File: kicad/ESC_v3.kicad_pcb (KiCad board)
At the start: 4 copper layers, 50 x 50 mm, 175 parts, among them J1 Conn_01x05_Pin, J2 Conn_01x05_Pin, J3 Conn_01x01_Pin, J4 Conn_01x06_Pin, J5 Conn_01x02_Pin, J6 Conn_01x06_Pin, J7 Conn_01x02_Pin, J8 Conn_01x04_Pin, J9 Conn_01x02_Pin, Q1 RH6L040BGTB1, Q10 RH6L040BGTB1, Q11 RH6L040BGTB1, Q12 RH6L040BGTB1, Q2 RH6L040BGTB1, Q3 RH6L040BGTB1, Q4 RH6L040BGTB1, Q5 RH6L040BGTB1, Q6 RH6L040BGTB1, Q7 RH6L040BGTB1, Q8 RH6L040BGTB1, Q9 RH6L040BGTB1, SW2 SW_Nidec_CAS-120A1, U1 L6387, U10 BD4104, U11 AMS1117-5.0, U12 ACS711xEXLT-15AB, U13 LM2937xMP, U14 MCP9700x-ETT, U15 MAX40200AUK, U19 STM32G431CBUx, U2 L6387, U3 L6387, U4 L6387, U5 L6387, U6 L6387, U7 AMS1117-3.3, U8 ACS711xEXLT-15AB, U9 ACS711xEXLT-15AB

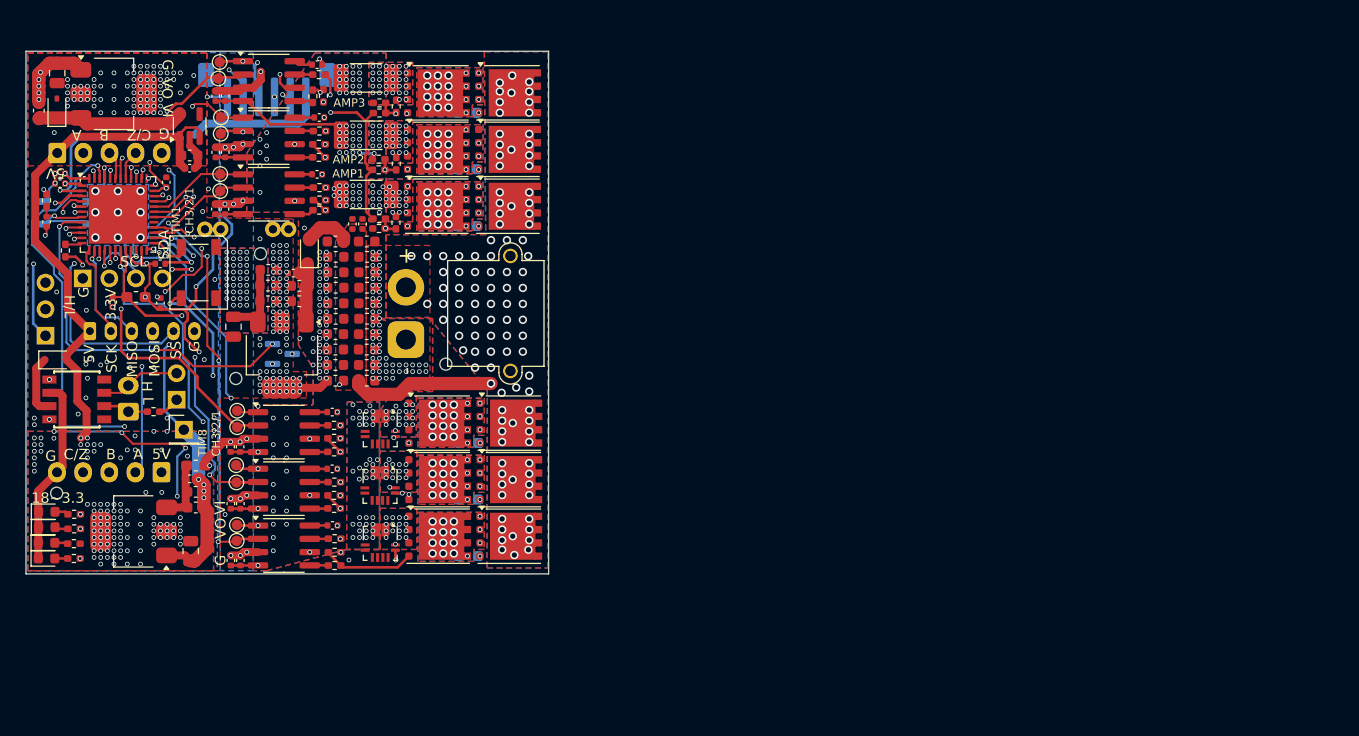
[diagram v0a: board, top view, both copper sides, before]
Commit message: a
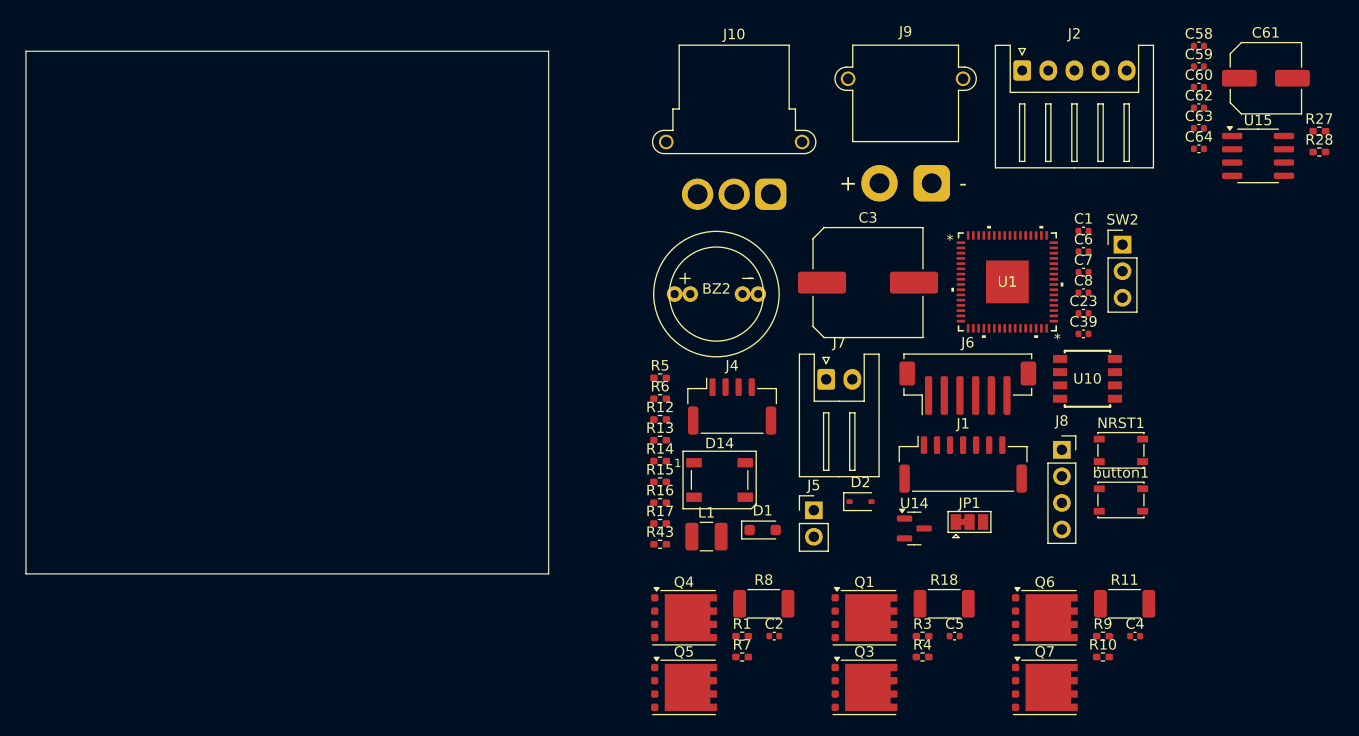
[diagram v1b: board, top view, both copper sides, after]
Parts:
- removed BZ1: Buzzer, jisaku:buzzer_unified
- removed C10, C12, C13, C15, C16, C18, C32, C38, C9: 0.1u, Capacitor_SMD:C_0402_1005Metric
- removed C11, C14, C17, C21, C33, C34, C35, C36, C37: 1u, Capacitor_SMD:C_0402_1005Metric
- removed C19, C20, C22: 10u, Capacitor_SMD:C_0603_1608Metric
- removed C24, C31, C40, C41, C42, C43, C44, C45, C46, C47, C48, C49, C50, C51, C52, C53, C54, C55, C56, C57: 22uF, Capacitor_SMD:C_0603_1608Metric
- removed C25, C29: 10uF, Capacitor_SMD:C_0603_1608Metric
- removed C26, C28, C30: 22uF, Capacitor_SMD:C_0805_2012Metric
- removed C27: 0.47uF, Capacitor_SMD:C_0603_1608Metric
- removed D13, D15, D16, D17: LED, LED_SMD:LED_0603_1608Metric
- removed D3: 1N5819WS, Diode_SMD:D_SOD-323
- removed G***: LOGO, agazou:full
- removed G***: LOGO, agazou:drive
- removed G***: LOGO, agazou:core
- removed G***: LOGO, agazou:blackpulsedrive
- removed J3: Conn_01x01_Pin, Connector_PinHeader_2.54mm:PinHeader_1x01_P2.54mm_Vertical
- removed L3: L, Inductor_SMD:L_0603_1608Metric_Pad1.05x0.95mm_HandSolder
- removed Q10, Q11, Q12, Q2, Q8, Q9: RH6L040BGTB1, Package_SON:VSONP-8-1EP_5x6_P1.27mm
- removed R19, R2, R20, R23, R24: 22, Resistor_SMD:R_0402_1005Metric_Pad0.72x0.64mm_HandSolder
- removed R21, R25, R57: 10k, Resistor_SMD:R_0402_1005Metric_Pad0.72x0.64mm_HandSolder
- removed R22, R26: 10k, Resistor_SMD:R_0603_1608Metric_Pad0.98x0.95mm_HandSolder
- removed R29: 100, Resistor_SMD:R_0402_1005Metric_Pad0.72x0.64mm_HandSolder
- removed R44, R45, R51: 5m, Resistor_SMD:R_2010_5025Metric_Pad1.40x2.65mm_HandSolder
- removed R46, R47, R52: 1.5k, Resistor_SMD:R_0402_1005Metric_Pad0.72x0.64mm_HandSolder
- removed R48, R49, R54: 68k, Resistor_SMD:R_0402_1005Metric_Pad0.72x0.64mm_HandSolder
- removed R50, R53, R55, R59: 2.2k, Resistor_SMD:R_0402_1005Metric_Pad0.72x0.64mm_HandSolder
- removed R56: 22k, Resistor_SMD:R_0402_1005Metric_Pad0.72x0.64mm_HandSolder
- removed R58: 4.7k, Resistor_SMD:R_0402_1005Metric_Pad0.72x0.64mm_HandSolder
- removed REF** (x4): ToolingHole_1.152mm, MountingHole:ToolingHole_1.152mm
- removed TP1, TP10, TP11, TP12, TP2, TP3, TP4, TP5, TP6, TP7, TP8, TP9: TestPoint, TestPoint:TestPoint_Pad_D1.0mm
- removed U11: AMS1117-5.0, Package_TO_SOT_SMD:SOT-223-3_TabPin2
- removed U12, U8, U9: ACS711xEXLT-15AB, Sensor_Current:Allegro_QFN-12-10-1EP_3x3mm_P0.5mm
- removed U13: LM2937xMP, Package_TO_SOT_SMD:SOT-223-3_TabPin2
- removed U19: STM32G431CBUx, Package_DFN_QFN:QFN-48-1EP_7x7mm_P0.5mm_EP5.6x5.6mm
- removed U2, U3, U4, U5, U6: L6387, Package_SO:SOIC-8_3.9x4.9mm_P1.27mm
- removed U7: AMS1117-3.3, Package_TO_SOT_SMD:SOT-223-3_TabPin2
- added BZ2: Buzzer, jisaku:buzzer_unified, F.Cu at (116.1, 73.2)
- added C39: 0.1u, Capacitor_SMD:C_0402_1005Metric, F.Cu at (151.2, 77.0)
- added C64: 10u, Capacitor_SMD:C_0402_1005Metric, F.Cu at (162.2, 59.3)
- added J10: Conn_01x03, Connector_AMASS:AMASS_MR30PW-FB_1x03_P3.50mm_Horizontal, F.Cu at (121.3, 63.7)
- added JP1: SolderJumper_3_Bridged12, Jumper:SolderJumper-3_P1.3mm_Bridged12_Pad1.0x1.5mm, F.Cu at (140.3, 95.0)
- added R27: 10k, Resistor_SMD:R_0402_1005Metric_Pad0.72x0.64mm_HandSolder, F.Cu at (173.7, 57.6)
- added R28: 10, Resistor_SMD:R_0402_1005Metric_Pad0.72x0.64mm_HandSolder, F.Cu at (173.7, 59.6)
- added R5: 10k, Resistor_SMD:R_0402_1005Metric_Pad0.72x0.64mm_HandSolder, F.Cu at (110.7, 81.2)
- added button1: SW_Push, Button_Switch_SMD:SW_SPST_PTS810, F.Cu at (154.8, 92.9)
- C1, C6, C7: value 0.1u -> 10u
- C3: value 0.1u -> 470u; footprint Capacitor_SMD:C_0402_1005Metric -> Capacitor_SMD:C_Elec_10x10.2
- C4: value 0.1u -> 1u
- C58: value 100u -> 4.7u; footprint Capacitor_SMD:C_0603_1608Metric -> Capacitor_SMD:C_0402_1005Metric
- C59: value 0.1u -> 0.033u
- C60: value 100u -> 0.05u; footprint Capacitor_SMD:C_0603_1608Metric -> Capacitor_SMD:C_0402_1005Metric
- C61: value 0.1u -> 470u; footprint Capacitor_SMD:C_0402_1005Metric -> Capacitor_SMD:C_Elec_6.3x7.7
- C62: value 100u -> 10u; footprint Capacitor_SMD:C_0603_1608Metric -> Capacitor_SMD:C_0402_1005Metric
- C8: value 1u -> 10u
- D1: value 1N5819WS -> D; footprint Diode_SMD:D_SOD-323 -> Diode_SMD:D_SOD-323_HandSoldering
- J1: value Conn_01x05_Pin -> Conn_01x07; footprint Connector_JST:JST_XH_S5B-XH-A_1x05_P2.50mm_Horizontal -> Connector_JST:JST_GH_SM07B-GHS-TB_1x07-1MP_P1.25mm_Horizontal; moved to F.Cu
- J2, J5, J6, J7, J8, NRST1, SW2, U14: moved to F.Cu
- J4: value Conn_01x06_Pin -> Conn_01x04; footprint Connector_JST:JST_PH_B6B-PH-K_1x06_P2.00mm_Vertical -> Connector_JST:JST_GH_SM04B-GHS-TB_1x04-1MP_P1.25mm_Horizontal; moved to F.Cu
- J9: value Conn_01x02_Pin -> Conn_01x02
- L1: value L -> 10uH; footprint Inductor_SMD:L_0603_1608Metric_Pad1.05x0.95mm_HandSolder -> Inductor_SMD:L_1210_3225Metric
- R1, R12, R15, R16, R7: value 22 -> R
- R10, R14, R4: value 10k -> R; footprint Resistor_SMD:R_0603_1608Metric_Pad0.98x0.95mm_HandSolder -> Resistor_SMD:R_0402_1005Metric_Pad0.72x0.64mm_HandSolder; moved to F.Cu
- R11, R8: value 22 -> R; footprint Resistor_SMD:R_0402_1005Metric_Pad0.72x0.64mm_HandSolder -> Resistor_SMD:R_2010_5025Metric
- R13, R17, R3, R9: value 10k -> R
- R18: value 10k -> R; footprint Resistor_SMD:R_0603_1608Metric_Pad0.98x0.95mm_HandSolder -> Resistor_SMD:R_2010_5025Metric; moved to F.Cu
- U1: value L6387 -> STSPIN32G4; footprint Package_SO:SOIC-8_3.9x4.9mm_P1.27mm -> stspin32g4:QFN_IN32G4_STM
- U15: value MAX40200AUK -> LM386; footprint Package_TO_SOT_SMD:SOT-23-5 -> Package_SO:SOIC-8_3.9x4.9mm_P1.27mm
- moved NRST1 103.4 mm to (154.8, 88.2), turned to 0 degrees
- moved SW2 103.4 mm to (154.9, 68.5)
- moved C61 103.3 mm to (168.6, 52.6)
- moved C62 102.8 mm to (162.2, 55.4)
- moved U15 102.3 mm to (167.9, 60.0), turned to 0 degrees
- moved C63 102.2 mm to (162.2, 57.4)
- moved C23 99.6 mm to (151.2, 75.1), turned to 0 degrees
- moved C60 96.8 mm to (162.2, 53.4)
- moved U10 96.7 mm to (151.6, 81.3)
- moved J8 95.1 mm to (149.1, 88.1), turned to 0 degrees
- moved J1 91.6 mm to (139.7, 89.5)
- moved J2 90.9 mm to (145.3, 51.8), turned to 0 degrees
- moved R11 89.3 mm to (155.1, 102.9)
- moved C58 89.1 mm to (162.2, 49.5), turned to 0 degrees
- moved C59 88.9 mm to (162.2, 51.5), turned to 0 degrees
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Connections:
- C1 pad 1: +12V -> Net-(U1-VCC)
- C2 pad 1: +12V -> /power_stage1/BOOT
- C2 pad 2: GND -> /power_stage1/OUT
- C3 pad 1: Net-(U1-VB) -> +15V
- C3 pad 2: /POWER/halfHbridge4/out1 -> OPAMP3_VINM
- C4 pad 1: +12V -> /power_stage2/BOOT
- C4 pad 2: GND -> /power_stage2/OUT
- C5 pad 1: +12V -> /power_stage/BOOT
- C5 pad 2: GND -> /power_stage/OUT
- C58 pad 1: Net-(D1-K) -> DAC1_OUT1
- C58 pad 2: GND -> Net-(C58-Pad2)
- C59 pad 1: Net-(D1-K) -> Net-(C59-Pad1)
- C59 pad 2: GND -> Net-(C59-Pad2)
- C6 pad 1: Net-(U2-VB) -> Net-(U1-REG3V3/VDD)
- C6 pad 2: /POWER/halfHbridge5/out1 -> GND
- C60 pad 1: +5V -> Net-(C59-Pad1)
- C60 pad 2: GND -> Net-(C60-Pad2)
- C61 pad 1: +5V -> Net-(C59-Pad1)
- C61 pad 2: GND -> /Untitled Sheet/OUT
- C62 pad 1: Net-(U11-VI) -> Net-(U15-BYPASS)
- C63 pad 1: Net-(U11-VI) -> /Untitled Sheet/VDD
- C7 pad 1: +12V -> +5V
- C8 pad 1: +12V -> Net-(U1-VCC)
- D1 pad 2: VCC -> GND
- J1 pad 1: +5V -> +3.3V
- J1 pad 2: TIM3_CH1 -> ADC1_IN8
- J1 pad 3: TIM3_CH2 -> GND
- J1 pad 4: EXTI13 -> ADC1_IN7
- J1 pad 5: GND -> unconnected-(J1-Pin_5-Pad5)
- J2 pad 1: +5V -> Net-(J2-Pin_1)
- J2 pad 2: TIM2_CH1 -> CH1
- J2 pad 3: TIM2_CH2 -> CH2
- J2 pad 4: TIM2_CH3 -> CH3
- J4 pad 1: +5V -> +3.3V
- J4 pad 2: SPI1_SCK -> ADC1_IN8
- J4 pad 3: SPI1_MISO -> GND
- J4 pad 4: SPI1_MOSI -> ADC1_IN7
- J9 pad 1: GND -> +15V
- J9 pad 2: VCC -> OPAMP3_VINP
- L1 pad 1: +3.3V -> Net-(D1-K)
- L1 pad 2: VREF -> Net-(U1-VCC)
- Q1 pad 1: /POWER/halfHbridge4/out1 -> /power_stage/OUT
- Q1 pad 3: VCC -> /power_stage/Vm
- Q3 pad 1: /POWER/halfHbridge5/out1 -> /power_stage/OPAMP_P
- Q3 pad 3: VCC -> /power_stage/OUT
- Q4 pad 1: /POWER/halfHbridge5/GND_mech -> /power_stage1/OUT
- Q4 pad 3: /POWER/halfHbridge5/out1 -> /power_stage/Vm
- Q5 pad 1: /POWER/halfHbridge6/out1 -> /power_stage1/OPAMP_P
- Q5 pad 3: VCC -> /power_stage1/OUT
- Q6 pad 1: /POWER/halfHbridge6/GND_mech -> /power_stage2/OUT
- Q6 pad 3: /POWER/halfHbridge6/out1 -> /power_stage/Vm
- Q7 pad 1: /POWER/halfHbridge7/out1 -> /power_stage2/OPAMP_P
- Q7 pad 3: VCC -> /power_stage2/OUT
- R1 pad 1: Net-(U1-HO) -> /power_stage1/GHS
- R1 pad 2: Net-(Q1-G) -> Net-(Q4-G)
- R10 pad 1: Net-(Q3-G) -> /power_stage2/GLS
- R10 pad 2: /POWER/halfHbridge5/out1 -> Net-(Q7-G)
- R11 pad 1: Net-(U3-HO) -> /power_stage2/OPAMP_P
- R11 pad 2: Net-(Q5-G) -> OPAMP3_VINM
- R12 pad 1: Net-(U3-LO) -> /power_stage/OPAMP_P
- R12 pad 2: Net-(Q6-G) -> OPAMP1_VINP
- R13 pad 1: /POWER/halfHbridge6/GND_mech -> OPAMP1_VINP
- R13 pad 2: Net-(Q6-G) -> +3.3V
- R14 pad 1: Net-(Q5-G) -> GND
- R14 pad 2: /POWER/halfHbridge6/out1 -> OPAMP1_VINP
- R15 pad 1: Net-(U4-HO) -> /power_stage1/OPAMP_P
- R15 pad 2: Net-(Q7-G) -> OPAMP2_VINP
- R16 pad 1: Net-(U4-LO) -> OPAMP2_VINP
- R16 pad 2: Net-(Q8-G) -> +3.3V
- R17 pad 1: /POWER/halfHbridge7/GND_mech -> GND
- R17 pad 2: Net-(Q8-G) -> OPAMP2_VINP
- R18 pad 1: Net-(Q7-G) -> /power_stage/OPAMP_P
- R18 pad 2: /POWER/halfHbridge7/out1 -> OPAMP3_VINM
- R3 pad 1: /POWER/halfHbridge4/GND_mech -> /power_stage/GLS
- R3 pad 2: Net-(Q2-G) -> Net-(Q3-G)
- R4 pad 1: Net-(Q1-G) -> /power_stage/GHS
- R4 pad 2: /POWER/halfHbridge4/out1 -> Net-(Q1-G)
- R7 pad 1: Net-(U2-HO) -> /power_stage1/GLS
- R7 pad 2: Net-(Q3-G) -> Net-(Q5-G)
- R8 pad 1: Net-(U2-LO) -> /power_stage1/OPAMP_P
- R8 pad 2: Net-(Q4-G) -> OPAMP3_VINM
- R9 pad 1: /POWER/halfHbridge5/GND_mech -> /power_stage2/GHS
- R9 pad 2: Net-(Q4-G) -> Net-(Q6-G)
- U1 pad 1: TIM1_CH1 -> Net-(U1-REG3V3/VDD)
- U1 pad 2: TIM1_CH1N -> Net-(U1-REG3V3/VDD)
- U1 pad 3: +12V -> unconnected-(U1-PC13-Pad3)
- U1 pad 4: GND -> unconnected-(U1-PC14-Pad4)
- U1 pad 5: Net-(U1-LO) -> unconnected-(U1-PC15-Pad5)
- U1 pad 6: /POWER/halfHbridge4/out1 -> RCC_HSE
- U1 pad 7: Net-(U1-HO) -> unconnected-(U1-PF1-Pad7)
- U1 pad 8: Net-(U1-VB) -> NRST
- U14 pad 2: ADC1_IN1 -> ADC1_IN9
- U15 pad 1: +5V -> Net-(R27-Pad1)
- U15 pad 3: +5V -> Net-(U15-+)
- U15 pad 4: unconnected-(U15-NC-Pad4) -> GND
- U15 pad 5: Net-(D3-K) -> Net-(C59-Pad1)
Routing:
- net GND: track 228.4 -> 0.00 mm, vias 340 -> 0
- net +3.3V: track 152.6 -> 0.00 mm, vias 94 -> 0
- net +5V: track 75.3 -> 0.00 mm, vias 104 -> 0
- net VREF: track 72.7 -> 0.00 mm, vias 6 -> 0
- net ADC2_IN10: track 66.5 -> 0.00 mm, vias 8 -> 0
- net +12V: track 56.0 -> 0.00 mm, vias 53 -> 0
- net TIM8_CH2: track 53.6 -> 0.00 mm, vias 5 -> 0
- net VCC: track 50.5 -> 0.00 mm, vias 110 -> 0
- net TIM8_CH1: track 47.1 -> 0.00 mm, vias 5 -> 0
- net ADC2_IN12: track 45.6 -> 0.00 mm, vias 3 -> 0
- net TIM8_CH1N: track 44.3 -> 0.00 mm, vias 5 -> 0
- net TIM8_CH2N: track 41.9 -> 0.00 mm, vias 4 -> 0
- net TIM8_CH3: track 40.6 -> 0.00 mm, vias 3 -> 0
- net OPAMP2_VINP: track 38.2 -> 0.00 mm, vias 4 -> 0
- net ADC1_IN11: track 35.7 -> 0.00 mm, vias 3 -> 0
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- removed copper zone on B.Cu, net +12V
- removed copper zone on F.Cu, net +12V
- removed copper zone on In1.Cu, net +12V
- removed copper zone on In2.Cu, net +12V
- removed copper zone on B.Cu, net +3.3V
- removed copper zone on F.Cu, net +3.3V
- removed copper zone on In1.Cu, net +3.3V
- removed copper zone on In2.Cu, net +3.3V
- removed copper zone on B.Cu, net +5V
- removed copper zone on F.Cu, net +5V
- removed copper zone on In1.Cu, net +5V
- removed copper zone on In2.Cu, net +5V
- removed copper zone on B.Cu, net /POWER/halfHbridge4/GND_mech
- removed copper zone on F.Cu, net /POWER/halfHbridge4/GND_mech
- removed copper zone on In1.Cu, net /POWER/halfHbridge4/GND_mech
- removed copper zone on In2.Cu, net /POWER/halfHbridge4/GND_mech
- removed copper zone on B.Cu, net /POWER/halfHbridge4/out1
- removed copper zone on F.Cu, net /POWER/halfHbridge4/out1
- removed copper zone on In1.Cu, net /POWER/halfHbridge4/out1
- removed copper zone on In2.Cu, net /POWER/halfHbridge4/out1
- removed copper zone on B.Cu, net /POWER/halfHbridge5/GND_mech
- removed copper zone on F.Cu, net /POWER/halfHbridge5/GND_mech
- removed copper zone on In1.Cu, net /POWER/halfHbridge5/GND_mech
- removed copper zone on In2.Cu, net /POWER/halfHbridge5/GND_mech
- removed copper zone on B.Cu, net /POWER/halfHbridge5/out1
- removed copper zone on F.Cu, net /POWER/halfHbridge5/out1
- removed copper zone on In1.Cu, net /POWER/halfHbridge5/out1
- removed copper zone on In2.Cu, net /POWER/halfHbridge5/out1
- removed copper zone on B.Cu, net /POWER/halfHbridge6/GND_mech
- removed copper zone on F.Cu, net /POWER/halfHbridge6/GND_mech
- removed copper zone on In1.Cu, net /POWER/halfHbridge6/GND_mech
- removed copper zone on In2.Cu, net /POWER/halfHbridge6/GND_mech
- removed copper zone on B.Cu, net /POWER/halfHbridge6/out1
- removed copper zone on F.Cu, net /POWER/halfHbridge6/out1
- removed copper zone on In1.Cu, net /POWER/halfHbridge6/out1
- removed copper zone on In2.Cu, net /POWER/halfHbridge6/out1
- removed copper zone on B.Cu, net /POWER/halfHbridge7/GND_mech
- removed copper zone on F.Cu, net /POWER/halfHbridge7/GND_mech
- removed copper zone on In1.Cu, net /POWER/halfHbridge7/GND_mech
- removed copper zone on In2.Cu, net /POWER/halfHbridge7/GND_mech
- removed copper zone on B.Cu, net /POWER/halfHbridge7/out1
- removed copper zone on F.Cu, net /POWER/halfHbridge7/out1
- removed copper zone on In1.Cu, net /POWER/halfHbridge7/out1
- removed copper zone on In2.Cu, net /POWER/halfHbridge7/out1
- removed copper zone on B.Cu, net /POWER/halfHbridge8/GND_mech
- removed copper zone on F.Cu, net /POWER/halfHbridge8/GND_mech
- removed copper zone on In1.Cu, net /POWER/halfHbridge8/GND_mech
- removed copper zone on In2.Cu, net /POWER/halfHbridge8/GND_mech
- removed copper zone on B.Cu, net /POWER/halfHbridge8/out1
- removed copper zone on F.Cu, net /POWER/halfHbridge8/out1
- removed copper zone on In1.Cu, net /POWER/halfHbridge8/out1
- removed copper zone on In2.Cu, net /POWER/halfHbridge8/out1
- removed copper zone on B.Cu, net /POWER/halfHbridge9/GND_mech
- removed copper zone on F.Cu, net /POWER/halfHbridge9/GND_mech
- removed copper zone on In1.Cu, net /POWER/halfHbridge9/GND_mech
- removed copper zone on In2.Cu, net /POWER/halfHbridge9/GND_mech
- removed copper zone on B.Cu, net /POWER/halfHbridge9/out1
- removed copper zone on F.Cu, net /POWER/halfHbridge9/out1
- removed copper zone on In1.Cu, net /POWER/halfHbridge9/out1
- removed copper zone on In2.Cu, net /POWER/halfHbridge9/out1
- removed copper zone on B.Cu, net GND
- removed copper zone on F.Cu, net GND
- removed copper zone on In1.Cu, net GND
- removed copper zone on In2.Cu, net GND
- removed copper zone on B.Cu, net VCC
- removed copper zone on F.Cu, net VCC
- removed copper zone on In1.Cu, net VCC
- removed copper zone on In2.Cu, net VCC
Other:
- board text removed: "18~3.3"
- board text removed: "3.3V"
- board text removed: "5V"
- board text removed: "A"
- board text removed: "AMP1"
- board text removed: "AMP2"
- board text removed: "AMP3"
- board text removed: "B"
- board text removed: "C/Z"
- board text removed: "CLK"
- board text removed: "DIO"
- board text removed: "G"
- board text removed: "GND"
- board text removed: "H"
- board text removed: "H/L"
- board text removed: "L"
- board text removed: "L/H"
- board text removed: "MISO"
- board text removed: "MOSI"
- board text removed: "NRST"
- board text removed: "RX"
- board text removed: "SCK"
- board text removed: "SCL"
- board text removed: "SDA"
- board text removed: "SS"
- board text removed: "TIM1 CH3/2/1"
- board text removed: "TIM8 CH3/2/1"
- board text removed: "TX"
- board text removed: "VI"
- board text removed: "VO"

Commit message: a
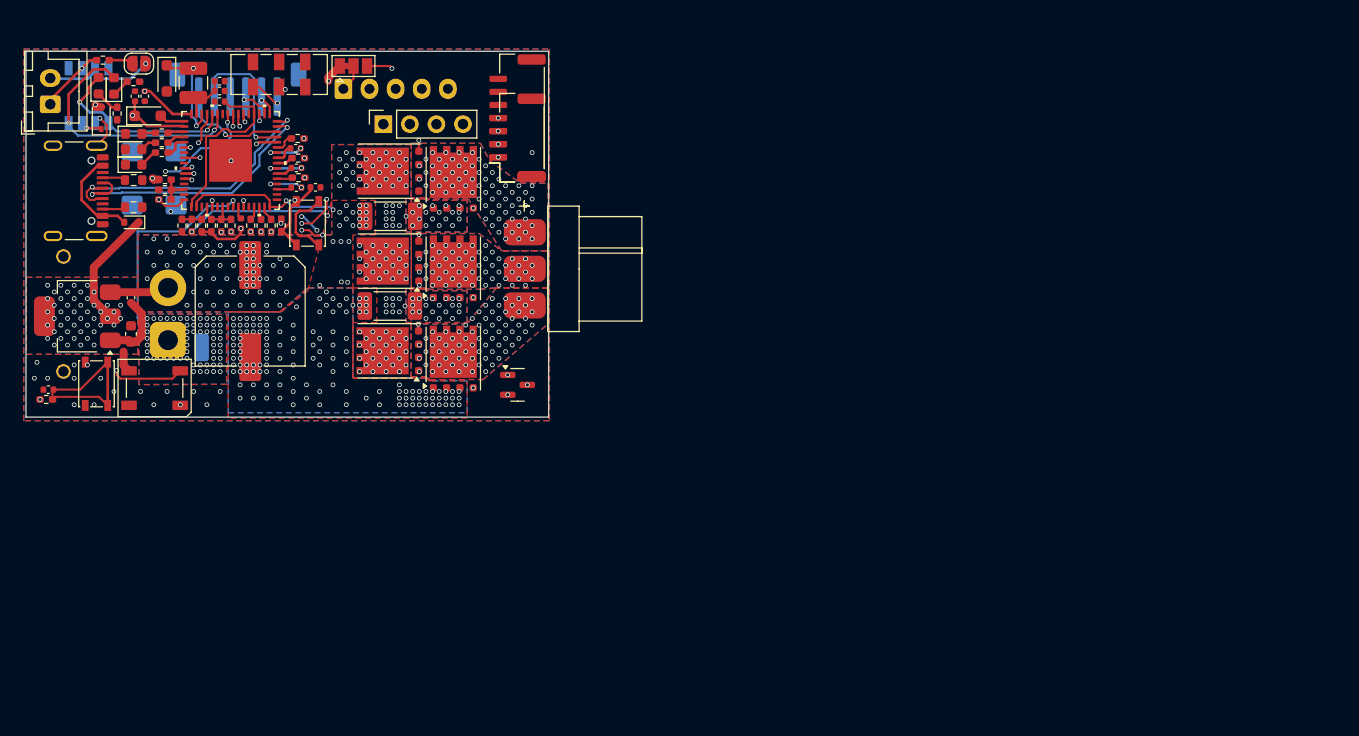
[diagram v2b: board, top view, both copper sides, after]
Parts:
- removed BZ2: Buzzer, jisaku:buzzer_unified
- removed C58: 4.7u, Capacitor_SMD:C_0402_1005Metric
- removed C59: 0.033u, Capacitor_SMD:C_0402_1005Metric
- removed C60: 0.05u, Capacitor_SMD:C_0402_1005Metric
- removed C61: 470u, Capacitor_SMD:C_Elec_6.3x7.7
- removed C62, C64: 10u, Capacitor_SMD:C_0402_1005Metric
- removed C63: 0.1u, Capacitor_SMD:C_0402_1005Metric
- removed J5: Conn_01x02_Pin, Connector_PinHeader_2.54mm:PinHeader_1x02_P2.54mm_Vertical
- removed R27: 10k, Resistor_SMD:R_0402_1005Metric_Pad0.72x0.64mm_HandSolder
- removed R28: 10, Resistor_SMD:R_0402_1005Metric_Pad0.72x0.64mm_HandSolder
- removed U15: LM386, Package_SO:SOIC-8_3.9x4.9mm_P1.27mm
- added C10: 10u, Capacitor_SMD:C_0402_1005Metric, F.Cu at (60.0, 73.6)
- added C11: 10u, Capacitor_SMD:C_0402_1005Metric, F.Cu at (68.5, 54.8)
- added C9: 22u, Capacitor_SMD:C_0603_1608Metric, F.Cu at (60.0, 77.0)
- added D3: 1N4148WT, Diode_SMD:D_SOD-523, F.Cu at (60.1, 66.4)
- added D4: LED_B, LED_SMD:LED_0603_1608Metric, F.Cu at (60.3, 57.9)
- added D5: LED_G, LED_SMD:LED_0603_1608Metric, F.Cu at (60.3, 59.4)
- added D6: LED_R, LED_SMD:LED_0603_1608Metric, F.Cu at (60.3, 60.9)
- added D7: D, Diode_SMD:D_SOD-323_HandSoldering, F.Cu at (61.6, 56.2)
- added D8: LED_R, LED_SMD:LED_0603_1608Metric, F.Cu at (58.4, 53.3)
- added D9: LED_G, LED_SMD:LED_0603_1608Metric, F.Cu at (56.9, 53.3)
- added J3: USB_C_Receptacle_USB2.0, Connector_USB:USB_C_Receptacle_GCT_USB4105-xx-A_16P_TopMnt_Horizontal, F.Cu at (53.7, 63.3)
- added JP2: SolderJumper_2_Open, Jumper:SolderJumper-2_P1.3mm_Open_RoundedPad1.0x1.5mm, F.Cu at (60.8, 51.2)
- added L2: L, Inductor_SMD:L_0402_1005Metric, F.Cu at (70.6, 66.5)
- added R19: R, Resistor_SMD:R_0402_1005Metric_Pad0.72x0.64mm_HandSolder, F.Cu at (63.3, 62.3)
- added R2: R, Resistor_SMD:R_2010_5025Metric_Pad1.40x2.65mm_HandSolder, B.Cu at (69.2, 78.3)
- added R20: R, Resistor_SMD:R_0402_1005Metric_Pad0.72x0.64mm_HandSolder, F.Cu at (63.3, 63.2)
- added R21: 2.2k, Resistor_SMD:R_0402_1005Metric_Pad0.72x0.64mm_HandSolder, F.Cu at (63.0, 59.7)
- added R22: 2.2k, Resistor_SMD:R_0402_1005Metric_Pad0.72x0.64mm_HandSolder, F.Cu at (63.0, 58.8)
- added R23: 5.1k, Resistor_SMD:R_0603_1608Metric, F.Cu at (60.3, 62.3)
- added R24: 5.1k, Resistor_SMD:R_0603_1608Metric, F.Cu at (60.3, 64.9)
- added R25: 2.2k, Resistor_SMD:R_0402_1005Metric_Pad0.72x0.64mm_HandSolder, F.Cu at (63.0, 57.8)
- added R26: 2.2k, Resistor_SMD:R_0402_1005Metric_Pad0.72x0.64mm_HandSolder, F.Cu at (60.3, 52.9)
- added R29: 2.2k, Resistor_SMD:R_0402_1005Metric_Pad0.72x0.64mm_HandSolder, F.Cu at (58.7, 56.0)
- added U2: AMS1117-5.0, Package_TO_SOT_SMD:SOT-223-3_TabPin2, F.Cu at (54.9, 75.3)
- added X1: IQXO-70, Oscillator:Oscillator_SMD_IQD_IQXO70-4Pin_7.5x5.0mm, B.Cu at (62.3, 62.2)
- J10: footprint Connector_AMASS:AMASS_MR30PW-FB_1x03_P3.50mm_Horizontal -> jisaku:MR30_side_SMD
- J2: footprint Connector_JST:JST_XH_S5B-XH-A_1x05_P2.50mm_Horizontal -> Connector_JST:JST_XH_B5B-XH-A_1x05_P2.50mm_Vertical; moved to B.Cu
- J6, J9, U10: moved to B.Cu
- J7: footprint Connector_JST:JST_XH_S2B-XH-A_1x02_P2.50mm_Horizontal -> Connector_JST:JST_XH_B2B-XH-A_1x02_P2.50mm_Vertical
- R11, R8: footprint Resistor_SMD:R_2010_5025Metric -> Resistor_SMD:R_2010_5025Metric_Pad1.40x2.65mm_HandSolder
- R18: footprint Resistor_SMD:R_2010_5025Metric -> Resistor_SMD:R_0402_1005Metric_Pad0.72x0.64mm_HandSolder
- SW2: footprint Connector_PinHeader_2.54mm:PinHeader_1x03_P2.54mm_Vertical -> Button_Switch_SMD:SW_DPDT_CK_JS202011JCQN
- moved U10 99.3 mm to (56.0, 54.2), turned to 90 degrees
- moved C39 99.2 mm to (52.1, 82.4), turned to 180 degrees
- moved button1 98.6 mm to (56.7, 81.8), turned to 90 degrees
- moved C6 92.0 mm to (60.4, 54.3), turned to 90 degrees
- moved C7 91.4 mm to (61.4, 54.3), turned to -90 degrees
- moved C4 91.0 mm to (75.9, 63.0)
- moved R10 89.6 mm to (73.5, 66.7), turned to -90 degrees
- moved R9 88.6 mm to (76.1, 62.1)
- moved C8 84.9 mm to (68.5, 53.8)
- moved R18 84.0 mm to (63.3, 64.2)
- moved C1 83.9 mm to (68.5, 52.9)
- moved SW2 82.3 mm to (74.2, 52.2), turned to 180 degrees
- moved D2 81.4 mm to (57.2, 56.4), turned to 90 degrees
- moved NRST1 80.8 mm to (76.9, 66.4), turned to -90 degrees
- moved J7 78.8 mm to (52.3, 55.1), turned to 90 degrees
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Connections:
- C3 pad 2: OPAMP3_VINM -> OPAMP1_VINM
- C6 pad 1: Net-(U1-REG3V3/VDD) -> +3.3V
- J9 pad 1: +15V -> OPAMP3_VINM
- J9 pad 2: OPAMP3_VINP -> +15V
- Q1 pad 3: /power_stage/Vm -> +15V
- Q3 pad 1: /power_stage/OPAMP_P -> /power_stage/GND
- Q4 pad 3: /power_stage/Vm -> +15V
- Q5 pad 1: /power_stage1/OPAMP_P -> /power_stage1/GND
- Q6 pad 3: /power_stage/Vm -> +15V
- Q7 pad 1: /power_stage2/OPAMP_P -> OPAMP1_VINM
- R11 pad 1: /power_stage2/OPAMP_P -> /power_stage1/GND
- R11 pad 2: OPAMP3_VINM -> OPAMP1_VINM
- R12 pad 1: /power_stage/OPAMP_P -> /power_stage/GND
- R15 pad 1: /power_stage1/OPAMP_P -> /power_stage1/GND
- R18 pad 1: /power_stage/OPAMP_P -> OPAMP1_VINM
- R18 pad 2: OPAMP3_VINM -> OPAMP3_VINP
- R8 pad 1: /power_stage1/OPAMP_P -> /power_stage/GND
- R8 pad 2: OPAMP3_VINM -> OPAMP1_VINM
- U1 pad 1: Net-(U1-REG3V3/VDD) -> Net-(D7-A)
- U1 pad 14: OPAMP1_VINP -> OPAMP3_VINP
- U1 pad 16: OPAMP3_VINM -> OPAMP1_VINM
- U1 pad 18: OPAMP2_VINP -> OPAMP1_VINM
- U1 pad 2: Net-(U1-REG3V3/VDD) -> +3.3V
- U1 pad 20: OPAMP3_VINM -> OPAMP1_VINP
- U1 pad 21: TX -> I2C_SCL
- U1 pad 22: RX -> unconnected-(U1-PC5-Pad22)
- U1 pad 23: OPAMP3_VINP -> OPAMP2_VINP
- U1 pad 26: unconnected-(U1-VREF+-Pad26) -> Net-(U1-VREF+)
- U1 pad 27: Net-(U1-REG3V3/VDD) -> +3.3V
- U1 pad 3: unconnected-(U1-PC13-Pad3) -> Net-(U1-PC13)
- U1 pad 32: OPAMP3_VINM -> OPAMP1_VINM
- U1 pad 4: unconnected-(U1-PC14-Pad4) -> Net-(U1-PC14)
- U1 pad 44: unconnected-(U1-PA8-Pad44) -> I2C_SDA
- U1 pad 45: unconnected-(U1-PA9-Pad45) -> TX
- U1 pad 46: unconnected-(U1-PA10-Pad46) -> RX
- U1 pad 49: I2C_SCL -> DIO
- U1 pad 5: unconnected-(U1-PC15-Pad5) -> Net-(U1-PC15)
- U1 pad 50: I2C_SDA -> CLK
- U1 pad 51: unconnected-(U1-PA15-Pad51) -> ToggleSwitch
- U1 pad 52: unconnected-(U1-SCREF-Pad52) -> DAC1_OUT1
- U1 pad 57: unconnected-(U1-PB6-Pad57) -> TIM4_CH2
- U1 pad 58: TIM4_CH2 -> unconnected-(U1-PB7-Pad58)
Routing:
- net +5V: track 0.00 -> 69.9 mm, vias 0 -> 51
- net ADC1_IN9: track 0.00 -> 62.9 mm, vias 0 -> 2
- net +3.3V: track 0.00 -> 57.7 mm, vias 0 -> 11
- net ADC1_IN8: track 0.00 -> 41.8 mm, vias 0 -> 2
- net ADC1_IN7: track 0.00 -> 39.9 mm, vias 0 -> 2
- net TIM4_CH2: track 0.00 -> 38.8 mm, vias 0 -> 3
- net OPAMP1_VINM: track 0.00 -> 38.2 mm, vias 0 -> 155
- net Net-(Q7-G): track 0.00 -> 31.4 mm, vias 0 -> 2
- net +15V: track 0.00 -> 30.1 mm, vias 0 -> 170
- net /power_stage2/OUT: track 0.00 -> 29.0 mm, vias 0 -> 76
- net USB_D+: track 0.00 -> 27.2 mm, vias 0 -> 2
- net OPAMP3_VINM: track 0.00 -> 26.8 mm, vias 0 -> 58
- net USB_D-: track 0.00 -> 26.5 mm, vias 0 -> 2
- net NRST: track 0.00 -> 26.3 mm, vias 0 -> 2
- net I2C_SCL: track 0.00 -> 26.0 mm, vias 0 -> 1
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- added copper zone on B.Cu, net +15V
- added copper zone on F.Cu, net +15V
- added copper zone on In1.Cu, net +15V
- added copper zone on In2.Cu, net +15V
- added copper zone on In3.Cu, net +15V
- added copper zone on In4.Cu, net +15V
- added copper zone on In2.Cu, net +3.3V
- added copper zone on In3.Cu, net +3.3V
- added copper zone on B.Cu, net +5V
- added copper zone on F.Cu, net +5V
- added copper zone on In1.Cu, net +5V
- added copper zone on In2.Cu, net +5V
- added copper zone on In3.Cu, net +5V
- added copper zone on In4.Cu, net +5V
- added copper zone on B.Cu, net /power_stage/GND
- added copper zone on F.Cu, net /power_stage/GND
- added copper zone on In1.Cu, net /power_stage/GND
- added copper zone on In2.Cu, net /power_stage/GND
- added copper zone on In3.Cu, net /power_stage/GND
- added copper zone on In4.Cu, net /power_stage/GND
- added copper zone on B.Cu, net /power_stage/OUT
- added copper zone on F.Cu, net /power_stage/OUT
- added copper zone on In1.Cu, net /power_stage/OUT
- added copper zone on In2.Cu, net /power_stage/OUT
- added copper zone on In3.Cu, net /power_stage/OUT
- added copper zone on In4.Cu, net /power_stage/OUT
- added copper zone on B.Cu, net /power_stage1/GND
- added copper zone on F.Cu, net /power_stage1/GND
- added copper zone on In1.Cu, net /power_stage1/GND
- added copper zone on In2.Cu, net /power_stage1/GND
- added copper zone on In3.Cu, net /power_stage1/GND
- added copper zone on In4.Cu, net /power_stage1/GND
- added copper zone on B.Cu, net /power_stage1/OUT
- added copper zone on F.Cu, net /power_stage1/OUT
- added copper zone on In1.Cu, net /power_stage1/OUT
- added copper zone on In2.Cu, net /power_stage1/OUT
- added copper zone on In3.Cu, net /power_stage1/OUT
- added copper zone on In4.Cu, net /power_stage1/OUT
- added copper zone on B.Cu, net /power_stage2/OUT
- added copper zone on F.Cu, net /power_stage2/OUT
- added copper zone on In1.Cu, net /power_stage2/OUT
- added copper zone on In2.Cu, net /power_stage2/OUT
- added copper zone on In3.Cu, net /power_stage2/OUT
- added copper zone on In4.Cu, net /power_stage2/OUT
- added copper zone on B.Cu, net GND
- added copper zone on F.Cu, net GND
- added copper zone on In1.Cu, net GND
- added copper zone on In4.Cu, net GND
- added copper zone on B.Cu, net OPAMP1_VINM
- added copper zone on F.Cu, net OPAMP1_VINM
- added copper zone on In1.Cu, net OPAMP1_VINM
- added copper zone on In2.Cu, net OPAMP1_VINM
- added copper zone on In3.Cu, net OPAMP1_VINM
- added copper zone on In4.Cu, net OPAMP1_VINM
- added copper zone on B.Cu, net OPAMP3_VINM
- added copper zone on F.Cu, net OPAMP3_VINM
- added copper zone on In1.Cu, net OPAMP3_VINM
- added copper zone on In2.Cu, net OPAMP3_VINM
- added copper zone on In3.Cu, net OPAMP3_VINM
- added copper zone on In4.Cu, net OPAMP3_VINM
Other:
- board size 50 x 50 mm -> 50 x 35 mm
- copper layers 4 -> 6
